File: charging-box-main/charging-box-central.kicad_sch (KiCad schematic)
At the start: 24 parts, among them J1 Accumulator 1, J10 mains power indicator, J11 Close AIRs, J2 Accumulator 2, J3 Main 12V, J4 Latching, J5 Charger, J6 IMD FAULT LED active low, J7 BMS LED active low, J8 Latching reset, J9 JESUS button, SW11 ON BUTTON

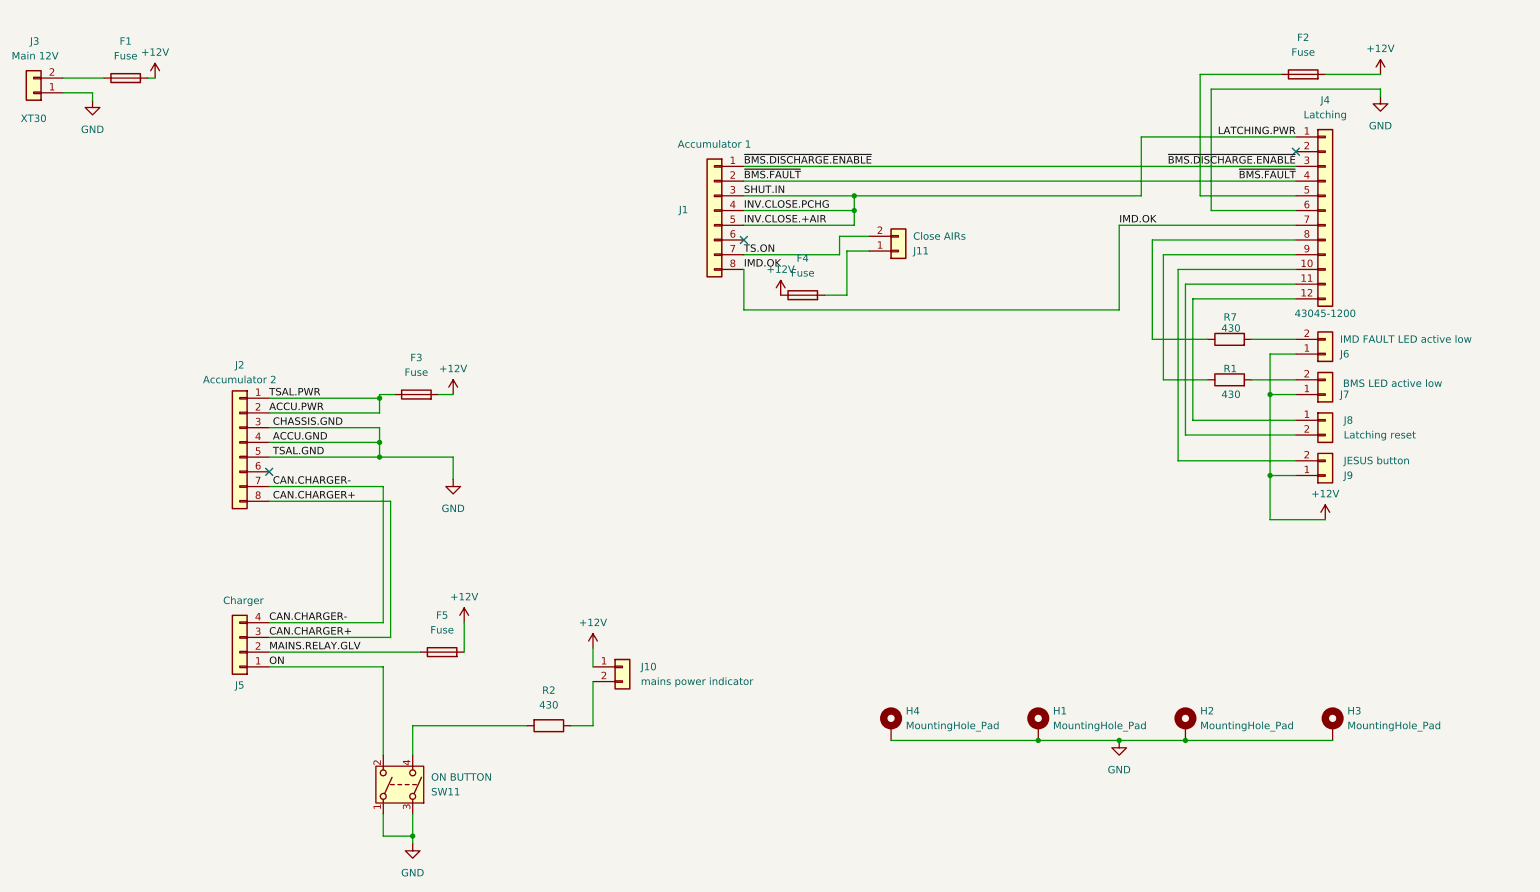
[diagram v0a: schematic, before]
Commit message: Changes
Production on pause
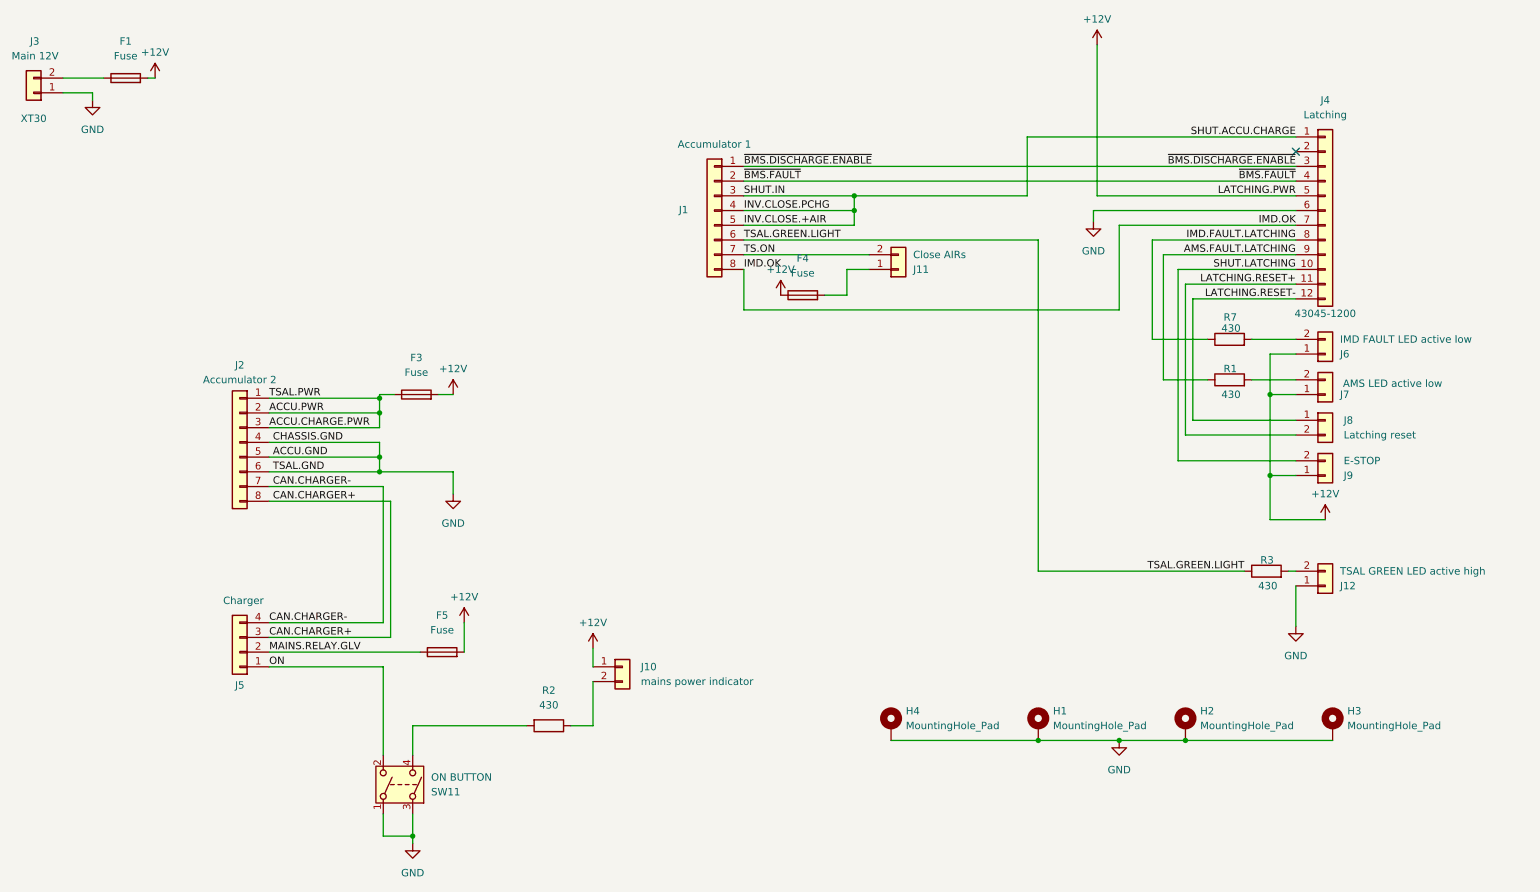
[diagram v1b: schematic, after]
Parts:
- removed F2: Fuse, Fuse:Fuse_0603_1608Metric, symbol Device:Fuse
- added J12: TSAL GREEN LED active high, Connector_Molex:Molex_Micro-Fit_3.0_43045-0200_2x01_P3.00mm_Horizontal, symbol Connector_Generic:Conn_01x02
- added R3: 430, Resistor_SMD:R_0805_2012Metric_Pad1.20x1.40mm_HandSolder, symbol Device:R
- J7: value BMS LED active low -> AMS LED active low
- J9: value JESUS button -> E-STOP
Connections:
- net +12V: now also J4.5 (Pin_5)
- net GND: now also J2.6 (Pin_6), J12.1 (Pin_1); no longer J2.3 (Pin_3)
- net LATCHING.RESET-: now reaches J4.12 (Pin_12), J8.1 (Pin_1)
- net LATCHING.RESET+: now reaches J4.11 (Pin_11), J8.2 (Pin_2)
- net SHUT.LATCHING: now reaches J4.10 (Pin_10), J9.2 (Pin_2)
- net IMD.FAULT.LATCHING: now reaches J4.8 (Pin_8), R7.1
- net AMS.FAULT.LATCHING: now reaches J4.9 (Pin_9), R1.1
- net TSAL.GREEN.LIGHT: now reaches J1.6 (Pin_6)
- net TSAL.GREEN.LIGHT: now also R3.1
- net ACCU.PWR renamed ACCU.CHARGE.PWR
- net ACCU.CHARGE.PWR: now also J2.3 (Pin_3)
- new net: J12.2 (Pin_2), R3.2
- no-connect marks 3 -> 1
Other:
- moved on the sheet: J11
